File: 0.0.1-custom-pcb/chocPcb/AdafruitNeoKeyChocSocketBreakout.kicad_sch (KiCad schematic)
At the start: 5 parts, among them J1 HC-FPC-0.5-6P-FH20, SW1 MX SOCKET

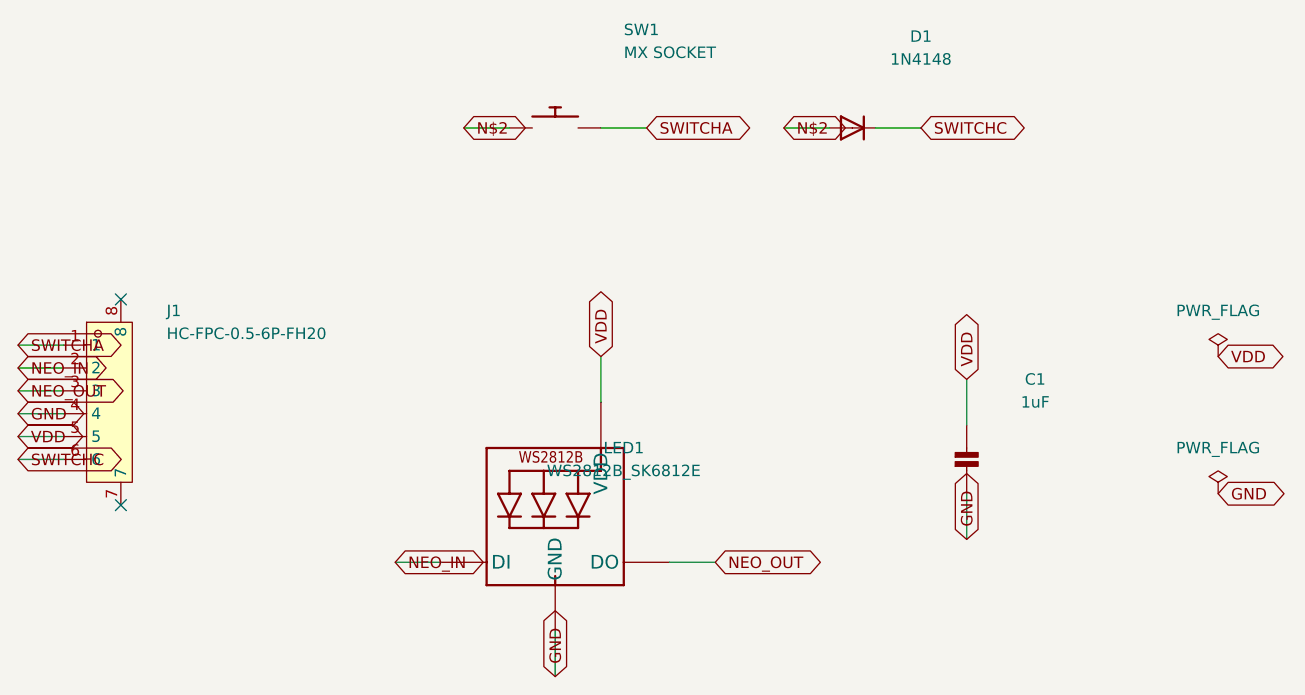
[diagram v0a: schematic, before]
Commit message: choc rev1 looking good!
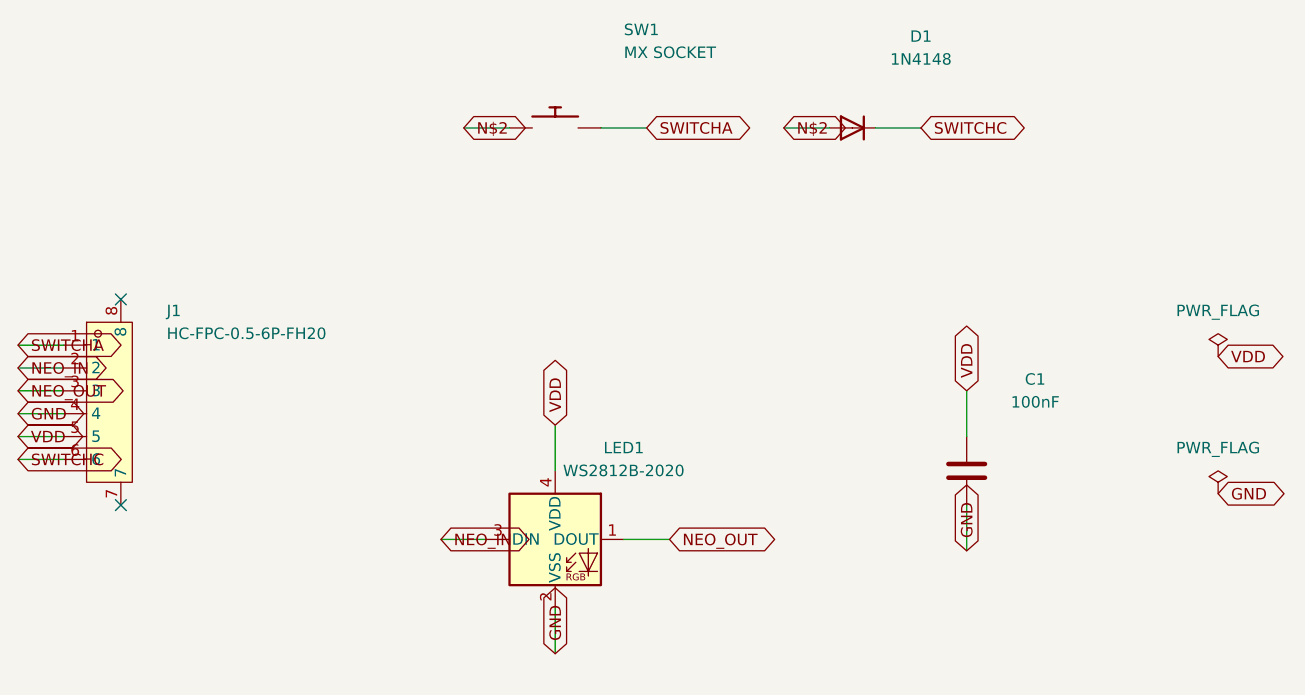
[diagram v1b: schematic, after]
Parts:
- C1: value 1uF -> 100nF; footprint AdafruitNeoKeyChocSocketBreakout:0603-NO -> ProjectParts:C_0402_1005Metric; symbol AdafruitNeoKeyChocSocketBreakout-eagle-import:CAP_CERAMIC0603_NO -> ProjectParts:C_0402_Decoupling; MPN (none) -> GRM155R71C104JA88D; Manufacturer (none) -> Murata; Substitution (none) -> Compatible replacement; exact Glove80 BOM not verified
- LED1: value WS2812B_SK6812E -> WS2812B-2020; footprint AdafruitNeoKeyChocSocketBreakout:NEO3535_REVERSE -> ProjectParts:LED_WS2812B-2020_PLCC4_2.0x2.0mm; symbol AdafruitNeoKeyChocSocketBreakout-eagle-import:WS2812B_SK6812E -> ProjectParts:WS2812B-2020; MPN (none) -> WS2812B-2020; Manufacturer (none) -> Worldsemi; Substitution (none) -> Compatible replacement; exact Glove80 BOM not verified
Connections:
- net GND: now also LED1.2 (VSS); no longer LED1.3-GND (GND)
- net NEO_IN: now also LED1.3 (DIN); no longer LED1.4-DIN (DI)
- net NEO_OUT: now also LED1.1 (DOUT); no longer LED1.2-DOUT (DO)
- net VDD: now also LED1.4 (VDD); no longer LED1.1-VDD (VDD)
